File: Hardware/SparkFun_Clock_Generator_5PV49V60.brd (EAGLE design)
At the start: 25.4 x 25.4 mm, 27 parts, among them U1 IDT_5P49V60_CLOCK_GENERATOR, Y2 26MHZ

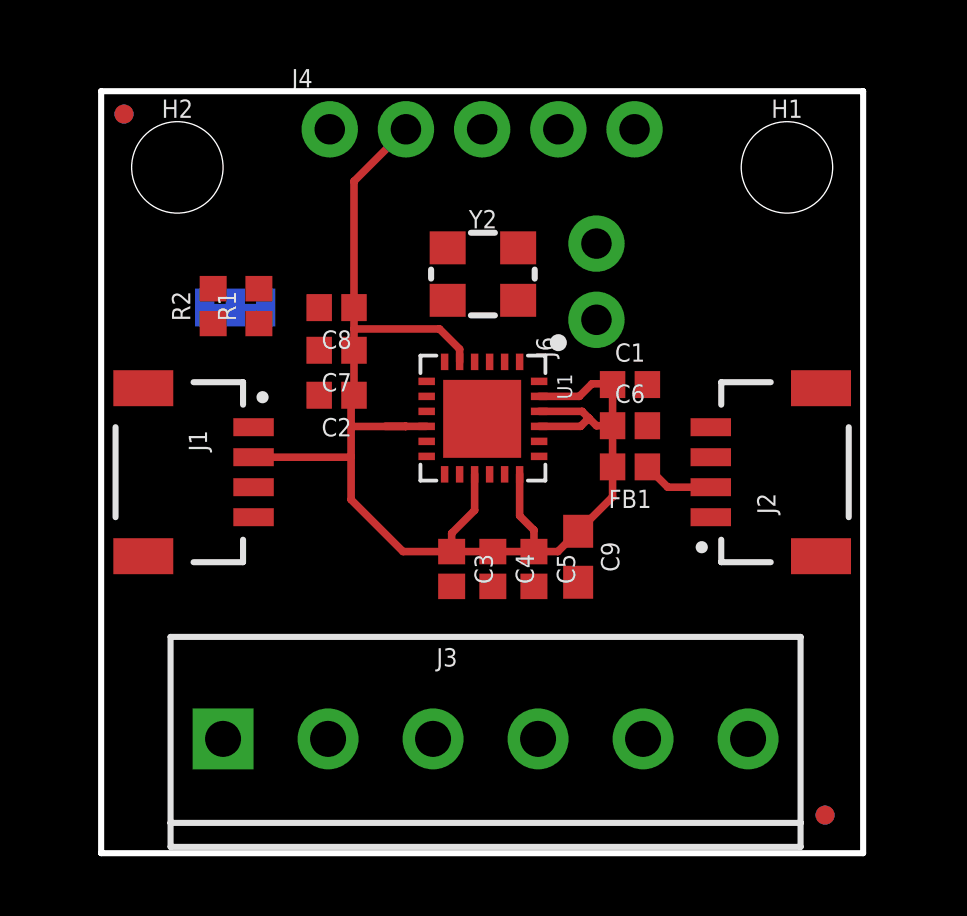
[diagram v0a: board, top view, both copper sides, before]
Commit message: Routes board
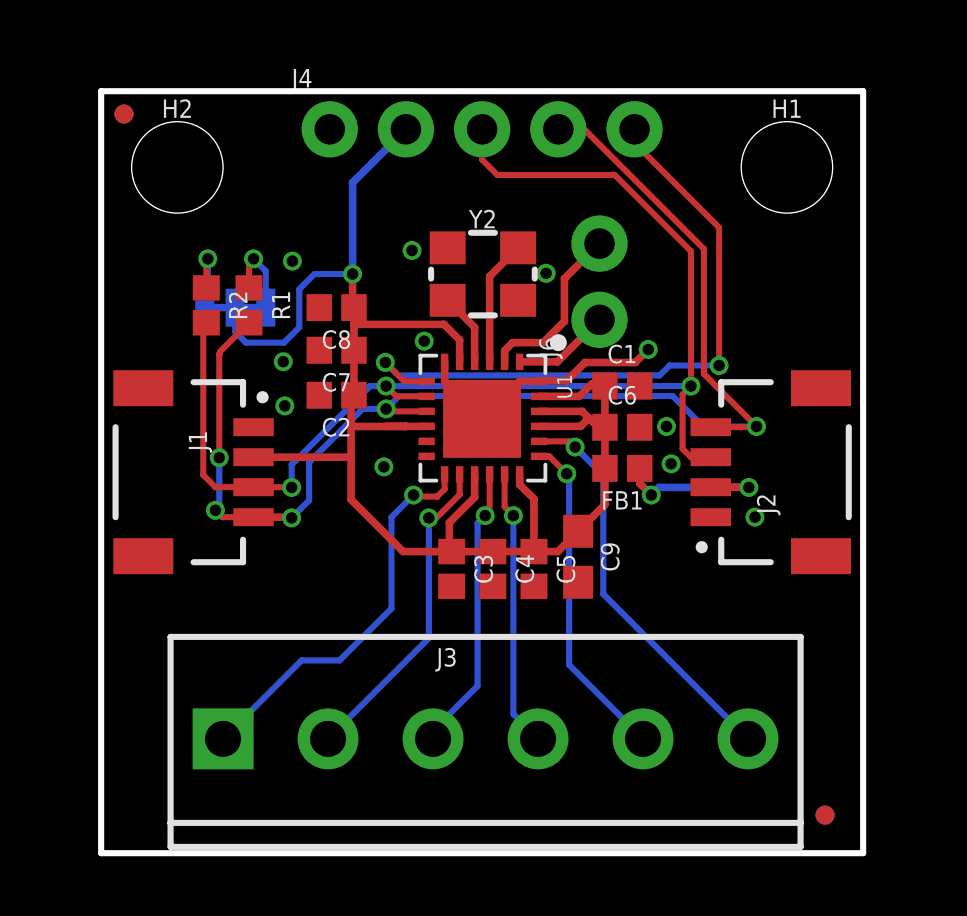
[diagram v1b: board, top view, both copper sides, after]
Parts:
- moved R1 0.33 mm to (4.93, 18.3), turned to 270 degrees
- moved C1 0.26 mm to (17.4, 15.6)
- moved FB1 0.26 mm to (17.4, 12.8)
- moved C6 0.26 mm to (17.4, 14.2)
- moved R2 0.23 mm to (3.51, 18.3), turned to 270 degrees
- moved J6 0.10 mm to (16.6, 17.8)
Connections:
- new net N$3: JP1.3, R1.1
- net SEL0/SCL: no longer JP1.3, R1.1
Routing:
- net SEL0/SCL: track 0.00 -> 43.8 mm, vias 0 -> 5
- net SEL1/SDA: track 0.00 -> 42.0 mm, vias 0 -> 3
- net SD/OE: track 0.00 -> 22.1 mm, vias 0 -> 2
- net OUT1: track 0.00 -> 13.8 mm, vias 0 -> 1
- net OUT3B: track 0.00 -> 13.2 mm, vias 0 -> 1
- net OUT1B: track 0.00 -> 11.1 mm, vias 0 -> 1
- net OUT3: track 0.00 -> 10.8 mm, vias 0 -> 1
- net OUT2B: track 0.00 -> 9.60 mm, vias 0 -> 1
- net 3.3V: track 53.5 -> 63.1 mm, vias 0 -> 3
- net OUT2: track 0.00 -> 9.28 mm, vias 0 -> 1
- net GND: track 0.00 -> 8.91 mm, vias 0 -> 11
- net CLKINB: track 0.00 -> 5.85 mm
- net N$4: track 0.00 -> 4.19 mm
- net CLKIN: track 0.00 -> 3.24 mm
- net N$3: track 0.00 -> 2.83 mm, vias 0 -> 1
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
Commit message: Adds silk, so much silk
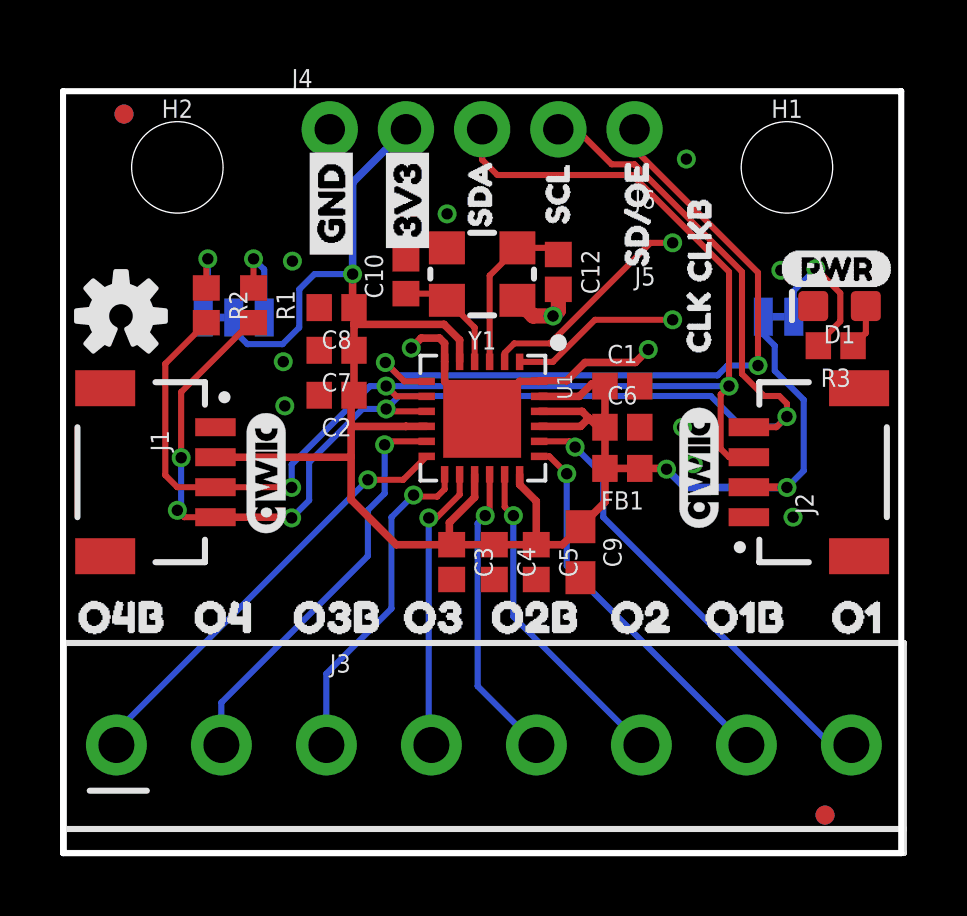
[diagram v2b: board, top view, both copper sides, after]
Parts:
- removed Y2: 26MHZ, SparkFun-Clocks:CRYSTAL-SMD-3.2X2.5MM
- added C10, C12: 12pF, SparkFun-Capacitors:0402
- added D1: RED, SparkFun-LED:LED-0603
- added J5: TEST-POINTTP_15TH_THRU, SparkFun-Connectors:TP_15TH
- added LED: JUMPER-SMT_2_NC_TRACE_SILK, SparkFun-Jumpers:SMT-JUMPER_2_NC_TRACE_SILK
- added LOGO1: SFE_LOGO_NAME_FLAME.1_INCH, SparkFun-Aesthetics:SFE_LOGO_NAME_FLAME_.1
- added LOGO2: OSHW-LOGOS, SparkFun-Aesthetics:OSHW-LOGO-S
- added LOGO3: QWIIC_LOGO_4MM, SparkFun-Aesthetics:QWIIC_4MM
- added R3: 1KOHM-0402-1/16W-1%, SparkFun-Resistors:0402
- added U$1: (no value), SparkFun-Aesthetics:QWIIC_4MM
- added U$10: (no value), Every Label:O29
- added U$11: (no value), Every Label:O2B10
- added U$12: (no value), Every Label:O37
- added U$13: (no value), Every Label:O3B8
- added U$14: (no value), Every Label:O4B6
- added U$15: (no value), Every Label:O45
- added U$16: (no value), Every Label:CLOCK_GENERATOR0
- added U$17: (no value), Every Label:5PV49V601
- added U$18, U$2: (no value), Labels:3V3-03
- added U$19, U$3: (no value), Labels:GND-03
- added U$20: (no value), Even more labels:OUT1B4
- added U$21: (no value), Even more labels:OUT2B6
- added U$22: (no value), Even more labels:OUT3B8
- added U$23: (no value), Even more labels:OUT4B10
- added U$24: (no value), Even more labels:OUT13
- added U$25: (no value), Even more labels:OUT25
- added U$26: (no value), Even more labels:OUT37
- added U$27: (no value), Even more labels:OUT49
- added U$28: (no value), Even more labels:SCL1
- added U$29: (no value), Even more labels:SD#OE2
- added U$30: (no value), Even more labels:SDA0
- added U$31, U$34: (no value), Even more labels:CLKB13
- added U$32: (no value), Even more labels:CLK11
- added U$33: (no value), Even more labels:CLK12
- added U$4: (no value), Labels:PWR-()-03
- added U$5: (no value), Every Label:SDA11
- added U$6: (no value), Every Label:SCL10
- added U$7: (no value), Every Label:SD#OE12
- added U$8: (no value), Every Label:O1B12
- added U$9: (no value), Every Label:O111
- added Y1: 16MHz, SparkFun-Clocks:CRYSTAL-SMD-3.2X2.5MM
- J3: device SparkFun-Connectors:SCREWTERMINAL-3.5MM-6 -> SparkFun-Connectors:SCREWTERMINAL-3.5MM-8
- J6: value (none) -> TEST-POINTTP_15TH_THRU; device SparkFun-Connectors:1X02_NO_SILK -> SparkFun-Connectors:TP_15TH
- moved J3 3.56 mm to (0.51, 3.61)
- moved J6 3.54 mm to (19.1, 20.3), turned to 0 degrees
- moved J1 1.27 mm to (3.81, 12.7)
- moved J2 1.27 mm to (21.6, 12.7)
- moved JP1 0.33 mm to (4.42, 17.9)
- moved C5 0.24 mm to (14.5, 9.70)
- moved C4 0.23 mm to (13.1, 9.70)
- moved C3 0.23 mm to (11.7, 9.70)
- moved C9 0.17 mm to (16.0, 10.0)
- moved R1 0.15 mm to (5.08, 18.3)
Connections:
- new net N$5: D1.A, R3.1
- new net N$6: C10.1, U1.P4, Y1.3
- net 3.3V: now also LED.2
- net CLKIN: now also J5.P$1; no longer J6.1
- net CLKINB: now also J6.P$1; no longer J6.2
- net GND: now also C10.2, C12.2, D1.C, Y1.2, Y1.4; no longer Y2.2, Y2.4
- net N$2: now also C12.1, U1.P3, Y1.1; no longer U1.P4, Y2.1
- net N$4: now also LED.1, R3.2; no longer U1.P3, Y2.3
- net OUT1: now also J3.8; no longer J3.6
- net OUT1B: now also J3.7; no longer J3.5
- net OUT2: now also J3.6; no longer J3.4
- net OUT2B: now also J3.5; no longer J3.3
- net OUT3: now also J3.4; no longer J3.2
- net OUT3B: now also J3.3; no longer J3.1
- net OUT4: now also J3.2
- net OUT4B: now also J3.1
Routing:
- net OUT4B: track 0.00 -> 14.6 mm, vias 0 -> 1
- net OUT4: track 0.00 -> 13.7 mm, vias 0 -> 1
- net 3.3V: track 63.1 -> 70.7 mm
- net GND: track 8.91 -> 13.2 mm, vias 11 -> 12
- net SEL1/SDA: track 42.0 -> 46.0 mm
- net N$6: track 0.00 -> 3.90 mm
- net SEL0/SCL: track 43.8 -> 47.4 mm
- net N$2: track 2.42 -> 5.64 mm
- net CLKIN: track 3.24 -> 5.68 mm
- net OUT3B: track 13.2 -> 11.2 mm
- net SD/OE: track 22.1 -> 24.0 mm
- net OUT1B: track 11.1 -> 12.8 mm
- net OUT1: track 13.8 -> 15.4 mm
- net OUT2: track 9.28 -> 10.9 mm
- net CLKINB: track 5.85 -> 7.42 mm
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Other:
- board size 25.4 x 25.4 mm -> 27.9 x 25.4 mm
- board text added: "Units in Inches"
